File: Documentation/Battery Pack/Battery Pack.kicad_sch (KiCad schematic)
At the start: 43 parts, among them K1 Air 1 GV200, K2 Air 2 GV200, P1 ASMPP30-1X2-KR, U4325RT1 BP1516, U4325RT10 BP1516, U4325RT11 BP1516, U4325RT12 BP1516, U4325RT13 BP1516, U4325RT14 BP1516, U4325RT15 BP1516, U4325RT16 BP1516, U4325RT17 BP1516, U4325RT18 BP1516, U4325RT19 BP1516, U4325RT2 BP1516, U4325RT20 BP1516, U4325RT21 BP1516, U4325RT22 BP1516, U4325RT23 BP1516, U4325RT24 BP1516, U4325RT25 BP1516, U4325RT26 BP1516, U4325RT27 BP1516, U4325RT28 BP1516, U4325RT29 BP1516, U4325RT3 BP1516, U4325RT30 BP1516, U4325RT31 BP1516, U4325RT32 BP1516, U4325RT33 BP1516, U4325RT34 BP1516, U4325RT4 BP1516, U4325RT5 BP1516, U4325RT6 BP1516, U4325RT7 BP1516, U4325RT8 BP1516, U4325RT9 BP1516, U4325RT? BP1516

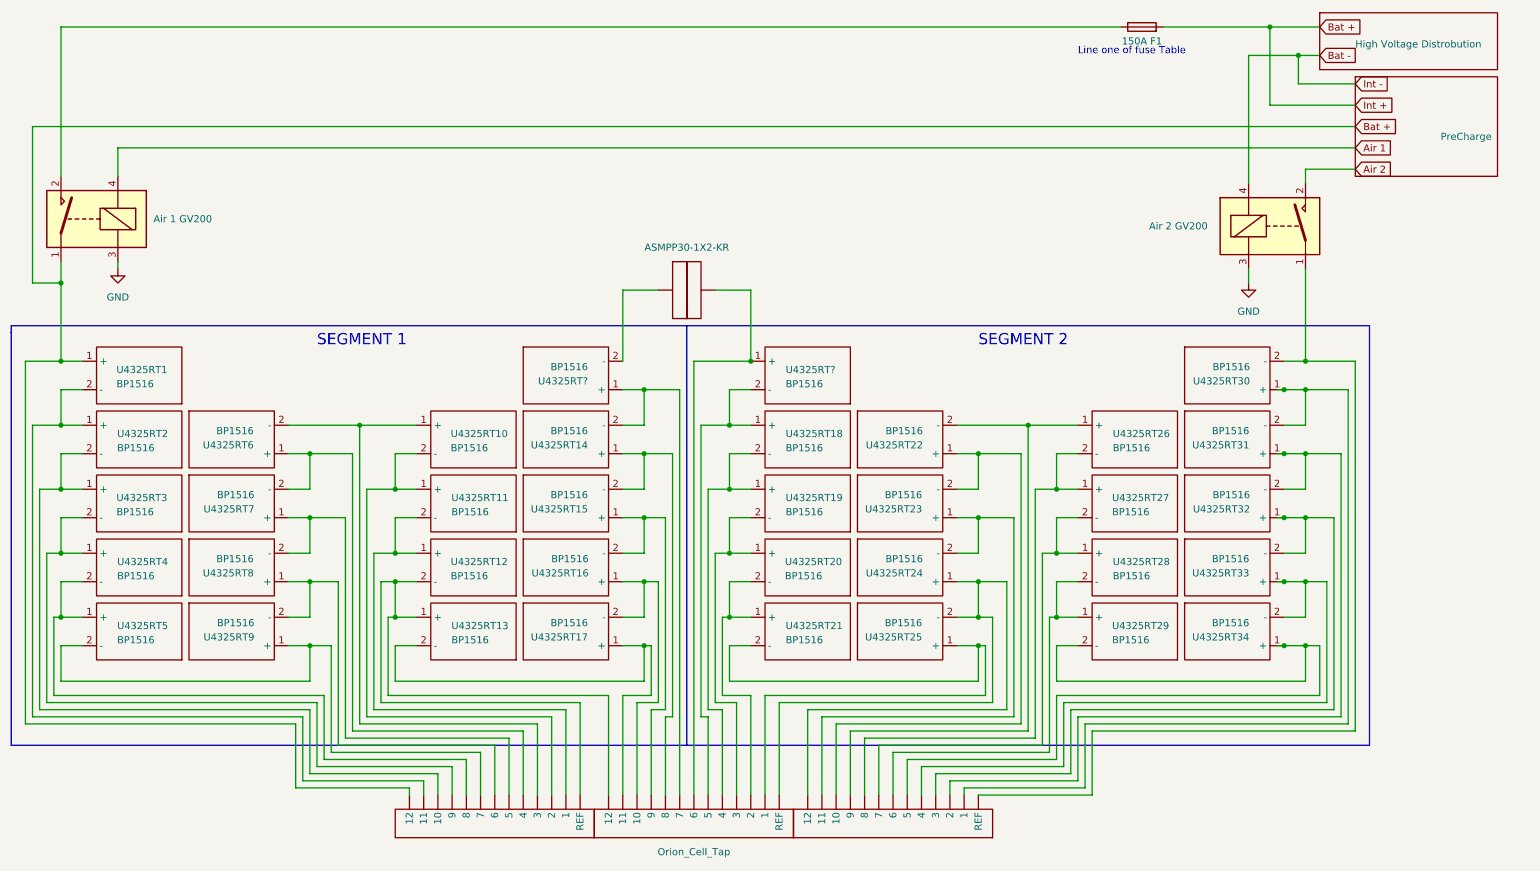
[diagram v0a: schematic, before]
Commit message: bat pac
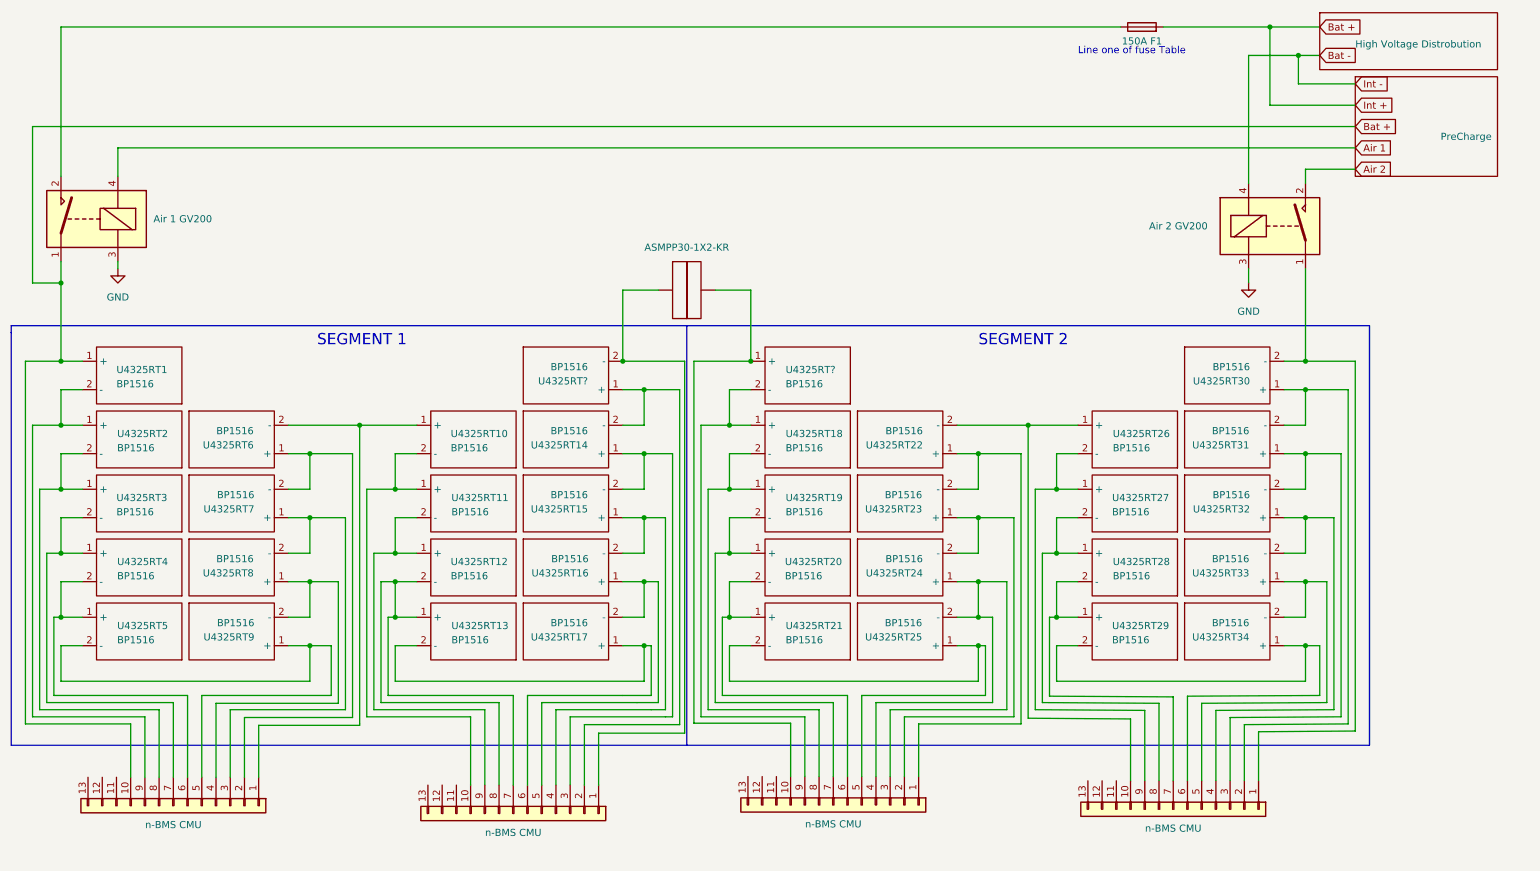
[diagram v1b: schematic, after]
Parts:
- removed U? (x3): Orion_Cell_Tap, symbol AERO_Symbols:Orion_Cell_Tap
- added J? (x4): n-BMS CMU, symbol Connector_Generic:Conn_01x13
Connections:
- net Bat +: now also J?.10 (Pin_10)
- net at U4325RT12.2 (-), U4325RT13.1 (+): now also J?.7 (Pin_7), J?.8 (Pin_8)
- net at U4325RT13.2 (-), U4325RT17.1 (+): now also J?.6 (Pin_6)
- net at U4325RT32.1 (+), U4325RT33.2 (-): now also J?.4 (Pin_4)
- net at U4325RT31.1 (+), U4325RT32.2 (-): now also J?.3 (Pin_3)
- net at U4325RT16.1 (+), U4325RT17.2 (-): now also J?.5 (Pin_5)
- net at U4325RT15.1 (+), U4325RT16.2 (-): now also J?.4 (Pin_4)
- net at U4325RT18.1 (+), U4325RT?.2 (-): now also J?.9 (Pin_9)
- net at U4325RT18.2 (-), U4325RT19.1 (+): now also J?.8 (Pin_8)
- net at U4325RT21.2 (-), U4325RT25.1 (+): now also J?.5 (Pin_5)
- net at U4325RT24.1 (+), U4325RT25.2 (-): now also J?.3 (Pin_3), J?.4 (Pin_4)
- net at U4325RT19.2 (-), U4325RT20.1 (+): now also J?.7 (Pin_7)
- net at U4325RT20.2 (-), U4325RT21.1 (+): now also J?.6 (Pin_6)
- net at U4325RT14.1 (+), U4325RT15.2 (-): now also J?.3 (Pin_3)
- net at P1., U4325RT?.1 (+): now also J?.10 (Pin_10)
- net at U4325RT14.2 (-), U4325RT?.1 (+): now also J?.2 (Pin_2)
- net at U4325RT6.1 (+), U4325RT7.2 (-): now also J?.2 (Pin_2)
- net at U4325RT10.1 (+), U4325RT6.2 (-): now also J?.1 (Pin_1)
- net at U4325RT3.2 (-), U4325RT4.1 (+): now also J?.7 (Pin_7)
- net at U4325RT4.2 (-), U4325RT5.1 (+): now also J?.6 (Pin_6)
- net at U4325RT8.1 (+), U4325RT9.2 (-): now also J?.4 (Pin_4)
- net at U4325RT7.1 (+), U4325RT8.2 (-): now also J?.3 (Pin_3)
- net at U4325RT22.2 (-), U4325RT26.1 (+): now also J?.10 (Pin_10)
- net at U4325RT26.2 (-), U4325RT27.1 (+): now also J?.9 (Pin_9)
- net at U4325RT27.2 (-), U4325RT28.1 (+): now also J?.8 (Pin_8)
- net at U4325RT28.2 (-), U4325RT29.1 (+): now also J?.7 (Pin_7)
- net at P1., U4325RT?.2 (-): now also J?.1 (Pin_1)
- net at U4325RT1.2 (-), U4325RT2.1 (+): now also J?.9 (Pin_9)
- net at U4325RT23.1 (+), U4325RT24.2 (-): now also J?.2 (Pin_2)
- net at U4325RT30.1 (+), U4325RT31.2 (-): now also J?.2 (Pin_2)
- net at U4325RT5.2 (-), U4325RT9.1 (+): now also J?.5 (Pin_5)
- net at U4325RT10.2 (-), U4325RT11.1 (+): now also J?.10 (Pin_10)
- net at U4325RT11.2 (-), U4325RT12.1 (+): now also J?.9 (Pin_9)
- net at U4325RT2.2 (-), U4325RT3.1 (+): now also J?.8 (Pin_8)
- net at U4325RT22.1 (+), U4325RT23.2 (-): now also J?.1 (Pin_1)
- net at K2.1, K2.14, U4325RT30.2 (-): now also J?.1 (Pin_1)
- net at U4325RT29.2 (-), U4325RT34.1 (+): now also J?.6 (Pin_6)
- net at U4325RT33.1 (+), U4325RT34.2 (-): now also J?.5 (Pin_5)

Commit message: end of year DUMP
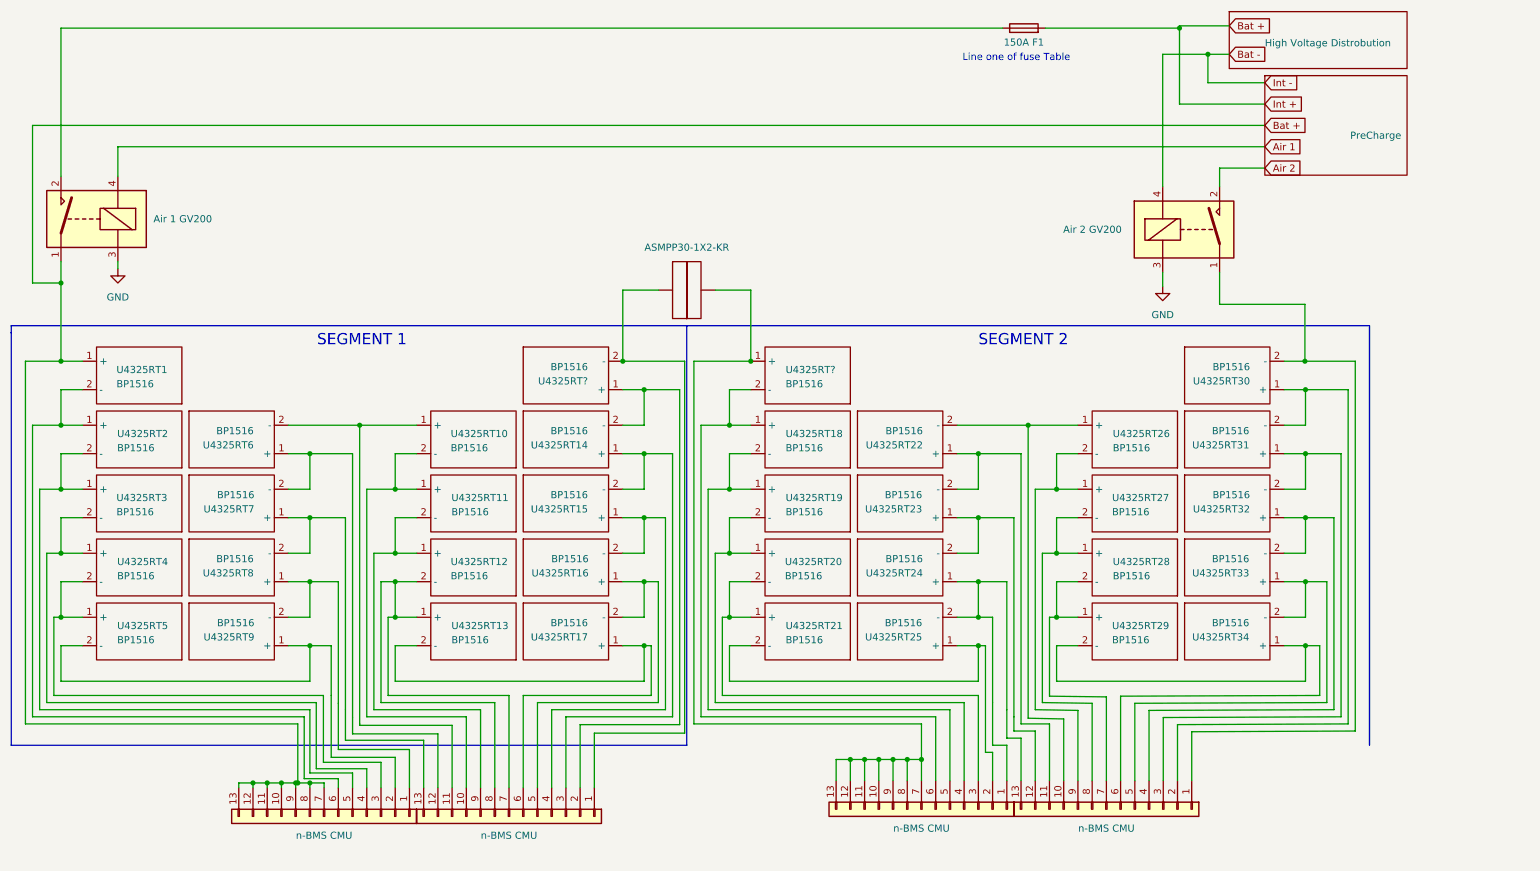
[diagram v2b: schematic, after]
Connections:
- net Bat +: now also J?.11 (Pin_11), J?.12 (Pin_12), J?.13 (Pin_13), J?.7 (Pin_7), J?.8 (Pin_8), J?.9 (Pin_9)
- net at U4325RT18.1 (+), U4325RT?.2 (-): now also J?.6 (Pin_6); no longer J?.9 (Pin_9)
- net at U4325RT18.2 (-), U4325RT19.1 (+): now also J?.5 (Pin_5); no longer J?.8 (Pin_8)
- net at U4325RT21.2 (-), U4325RT25.1 (+): now also J?.2 (Pin_2); no longer J?.5 (Pin_5)
- net at U4325RT24.1 (+), U4325RT25.2 (-): now also J?.1 (Pin_1), J?.13 (Pin_13); no longer J?.3 (Pin_3), J?.4 (Pin_4)
- net at U4325RT6.1 (+), U4325RT7.2 (-): now also J?.12 (Pin_12); no longer J?.2 (Pin_2)
- net at U4325RT10.1 (+), U4325RT6.2 (-): now also J?.11 (Pin_11); no longer J?.1 (Pin_1)
- net at U4325RT3.2 (-), U4325RT4.1 (+): now also J?.4 (Pin_4); no longer J?.7 (Pin_7)
- net at U4325RT4.2 (-), U4325RT5.1 (+): now also J?.3 (Pin_3); no longer J?.6 (Pin_6)
- net at U4325RT19.2 (-), U4325RT20.1 (+): now also J?.4 (Pin_4); no longer J?.7 (Pin_7)
- net at U4325RT20.2 (-), U4325RT21.1 (+): now also J?.3 (Pin_3); no longer J?.6 (Pin_6)
- net at U4325RT8.1 (+), U4325RT9.2 (-): now also J?.1 (Pin_1); no longer J?.4 (Pin_4)
- net at U4325RT7.1 (+), U4325RT8.2 (-): now also J?.13 (Pin_13); no longer J?.3 (Pin_3)
- net at J?.10 (Pin_10), P1., U4325RT?.1 (+): now also J?.11 (Pin_11), J?.12 (Pin_12), J?.13 (Pin_13), J?.7 (Pin_7), J?.8 (Pin_8), J?.9 (Pin_9)
- net at J?.11 (Pin_11): now also U4325RT22.1 (+), U4325RT23.2 (-)
- net at J?.12 (Pin_12): now also U4325RT23.1 (+), U4325RT24.2 (-)
- net at U4325RT1.2 (-), U4325RT2.1 (+): now also J?.6 (Pin_6); no longer J?.9 (Pin_9)
- net at U4325RT5.2 (-), U4325RT9.1 (+): now also J?.2 (Pin_2); no longer J?.5 (Pin_5)
- net at U4325RT2.2 (-), U4325RT3.1 (+): now also J?.5 (Pin_5); no longer J?.8 (Pin_8)
